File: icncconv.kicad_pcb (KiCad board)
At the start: 4 copper layers, 82.9 x 50 mm, 60 parts, among them J1 Conn_01x11_Pin, J3 Conn_01x11_Pin, SW1 SS-3292S-L2-B, U1 iC-NV, U2 MC3487N

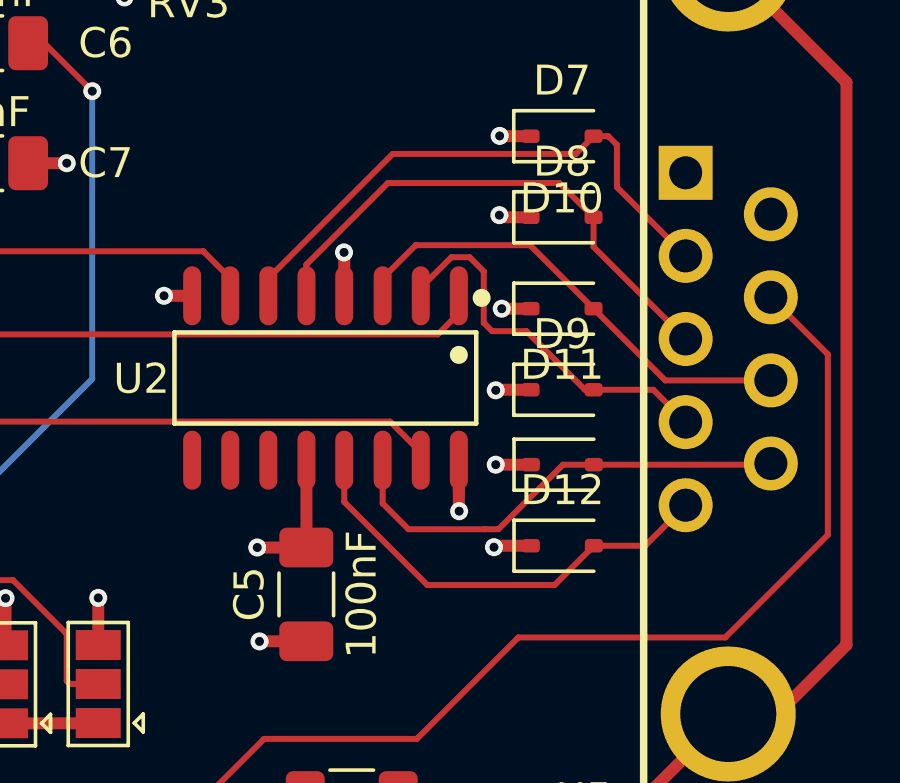
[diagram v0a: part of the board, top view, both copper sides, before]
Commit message: up
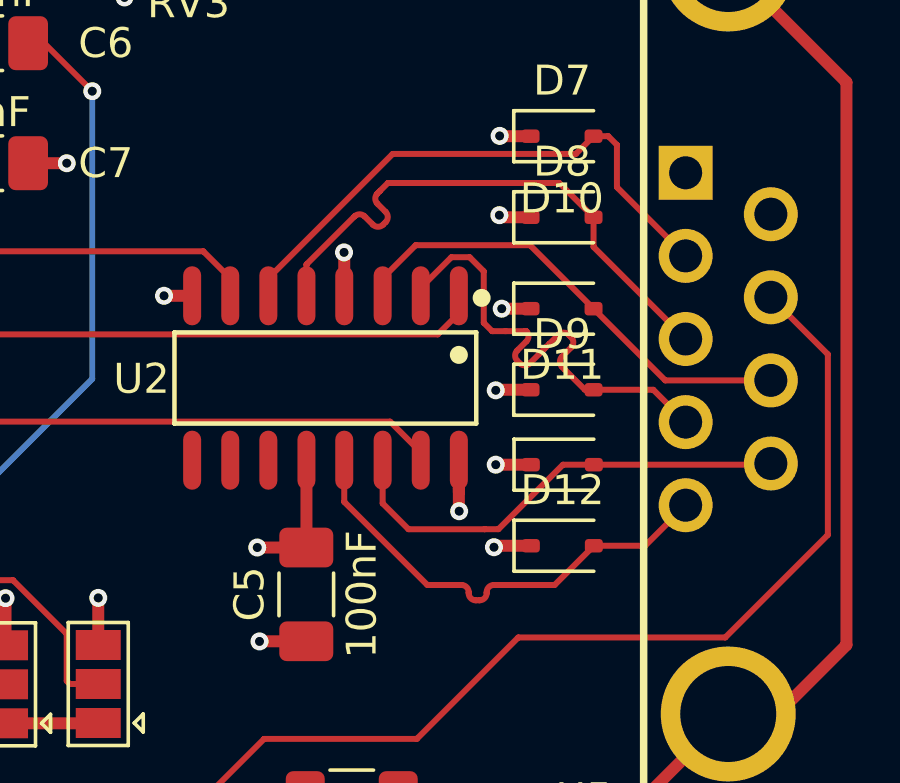
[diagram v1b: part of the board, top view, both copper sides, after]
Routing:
- net B+: track 12.8 -> 15.8 mm
- net A-: track 17.5 -> 18.8 mm
- net Z-: track 15.0 -> 15.6 mm

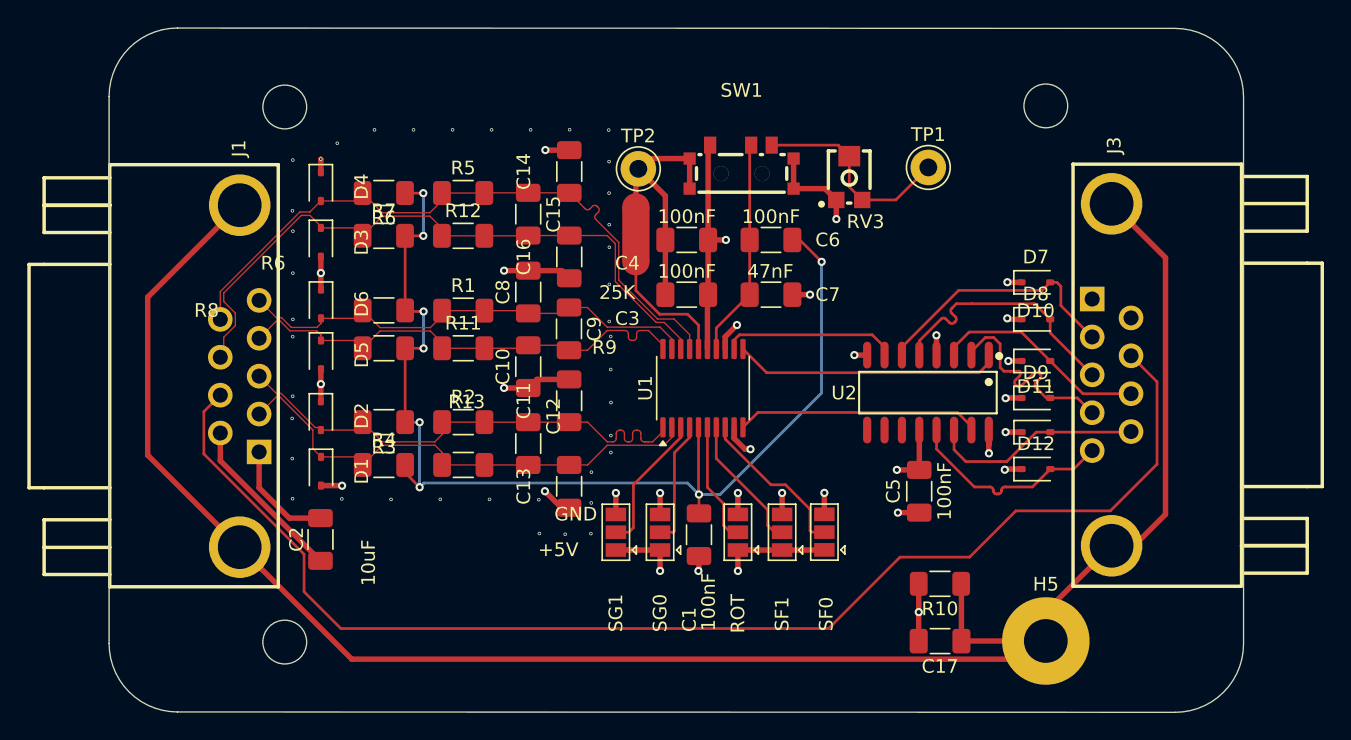
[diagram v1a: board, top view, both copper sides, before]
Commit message: update
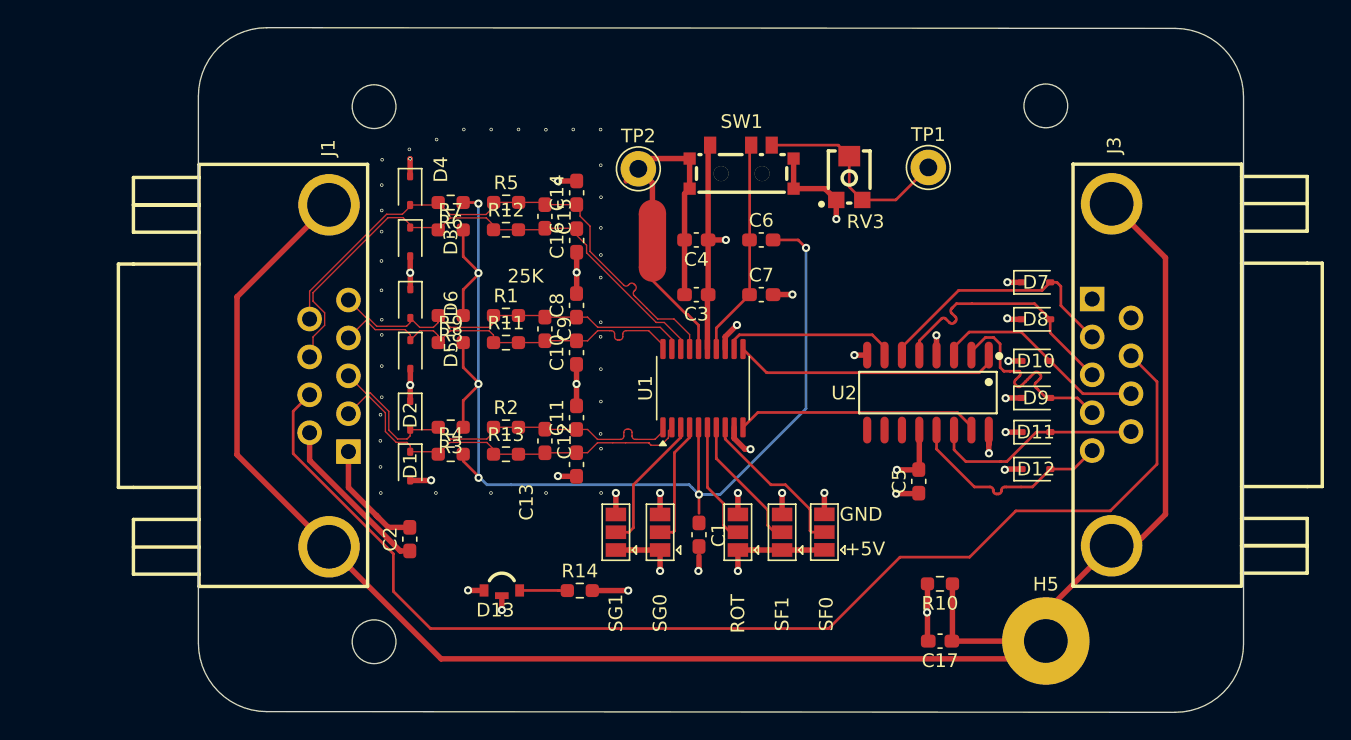
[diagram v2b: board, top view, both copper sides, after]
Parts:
- added D13: LED, easyeda2kicad:LED-SMD_L3.2-W1.0-R-RD_GREEN, F.Cu at (136.7, 116.3)
- added R14: 150, Resistor_SMD:R_0603_1608Metric_Pad0.98x0.95mm_HandSolder, F.Cu at (142.4, 116.1)
- C1, C10, C11, C12, C13, C14, C15, C16, C17, C2, C3, C4, C5, C6, C7, C8, C9: footprint Capacitor_SMD:C_1206_3216Metric_Pad1.33x1.80mm_HandSolder -> Capacitor_SMD:C_0603_1608Metric_Pad1.08x0.95mm_HandSolder
- R1, R10, R11, R12, R13, R2, R3, R4, R5, R6, R7, R8, R9: footprint Resistor_SMD:R_1206_3216Metric_Pad1.30x1.75mm_HandSolder -> Resistor_SMD:R_0603_1608Metric_Pad0.98x0.95mm_HandSolder
- moved D1 6.53 mm to (130.0, 107.0)
- moved C2 6.53 mm to (130.0, 112.4)
- moved D2 6.53 mm to (130.0, 103.3)
- moved D3 6.53 mm to (130.0, 90.6)
- moved D5 6.53 mm to (130.0, 98.9)
- moved D6 6.53 mm to (130.0, 95.2)
- moved H1 6.53 mm to (127.4, 80.8)
- moved H3 6.53 mm to (127.4, 119.9)
- moved J1 6.53 mm to (124.1, 100.4)
- moved D4 6.53 mm to (130.0, 86.9)
- moved R4 4.95 mm to (133.0, 106.2)
- moved R6 4.94 mm to (133.0, 87.8)
- moved R7 4.91 mm to (133.0, 89.8)
- moved R9 4.90 mm to (133.0, 98.0)
- moved R3 4.90 mm to (133.0, 104.2)
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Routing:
- net IDX-: track 49.0 -> 40.8 mm
- net IDX+: track 48.9 -> 40.7 mm
- net COS-: track 36.9 -> 29.2 mm
- net COS+: track 36.8 -> 29.2 mm
- net SIN+: track 34.9 -> 28.3 mm
- net SIN-: track 34.9 -> 28.3 mm
- net SHIELD: track 95.1 -> 88.5 mm
- net GNDS: track 142.0 -> 138.0 mm
- net ICNV_VREF: track 81.6 -> 85.5 mm, vias 8 -> 6
- net Net-(D13-K): track 0.00 -> 3.49 mm
- net GNDA: track 9.48 -> 7.37 mm
- net +5V: track 51.4 -> 52.2 mm, vias 7 -> 8
- net GND: track 81.5 -> 80.7 mm
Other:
- board size 82.9 x 50 mm -> 76.4 x 50.1 mm
- board text removed: "R6"

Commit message: update prodv1
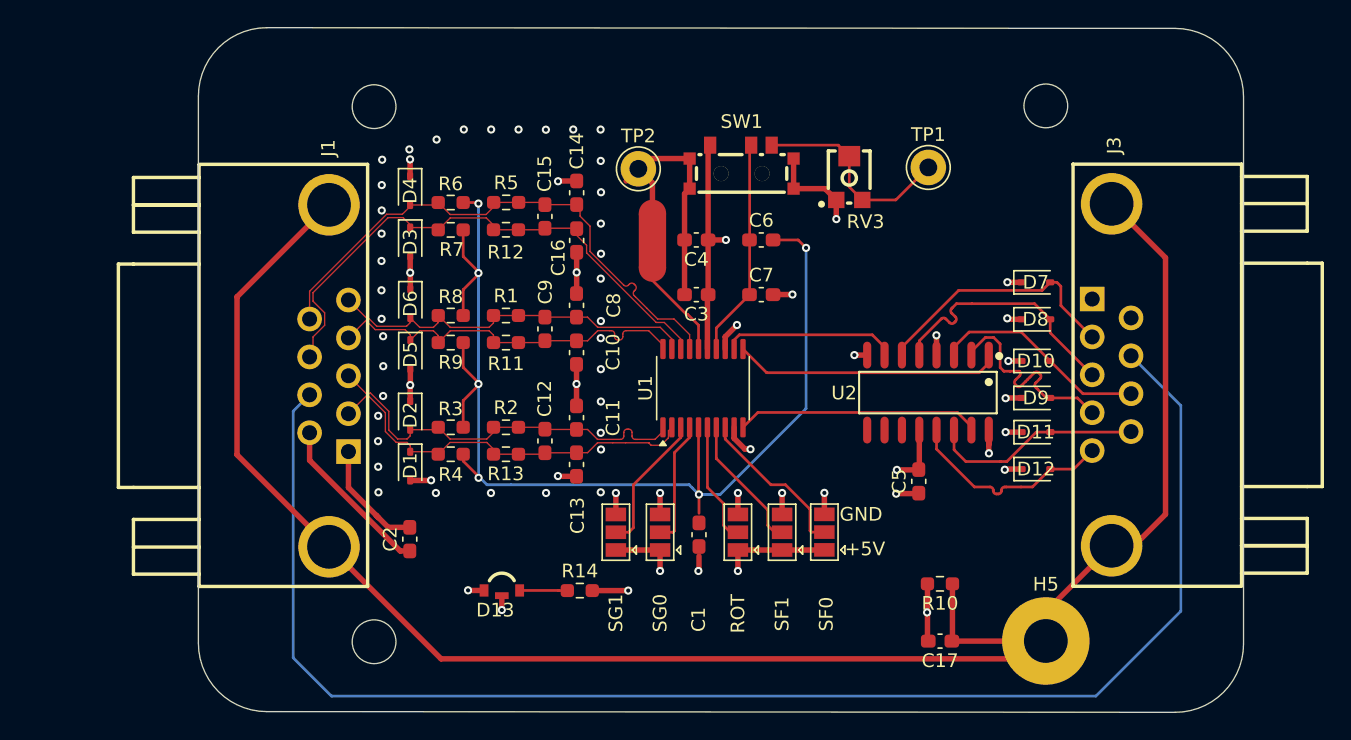
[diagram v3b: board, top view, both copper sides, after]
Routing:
- net SHIELD: track 88.5 -> 108.5 mm
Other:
- board text removed: "25K"
